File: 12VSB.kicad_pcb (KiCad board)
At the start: 4 copper layers, 24 parts, among them U1 FP6296

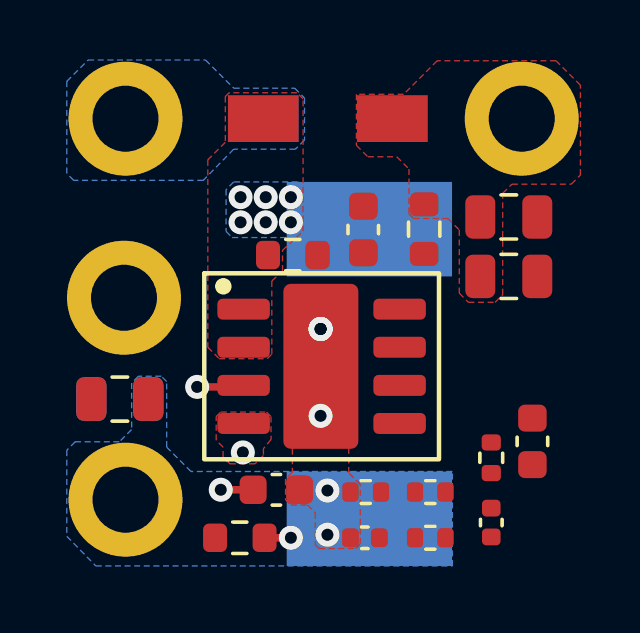
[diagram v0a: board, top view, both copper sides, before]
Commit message: Updated PCB Layout and Documentation
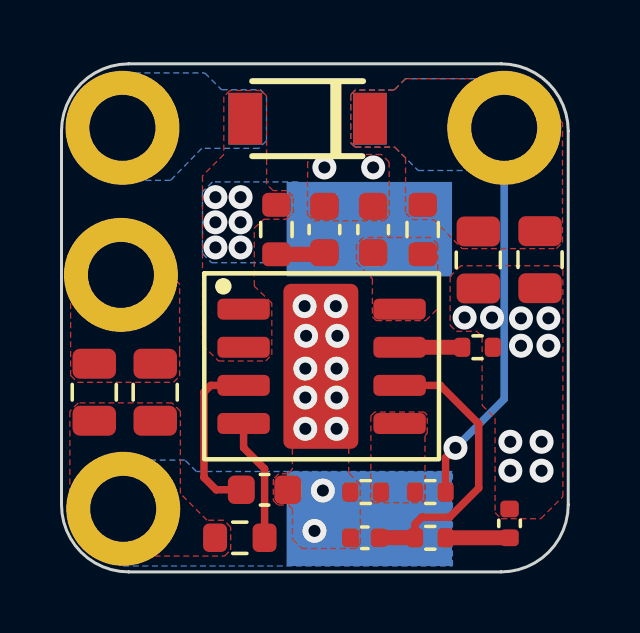
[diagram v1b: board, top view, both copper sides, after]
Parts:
- C2: moved to F.Cu
- moved C9 8.83 mm to (63.1, 58.1)
- moved R3 3.71 mm to (66.6, 62.0), turned to 0 degrees
- moved C5 1.76 mm to (68.7, 59.1), turned to -90 degrees
- moved C12 1.30 mm to (61.5, 58.1)
- moved C2 1.20 mm to (55.9, 63.5), turned to 90 degrees
- moved C6 1.15 mm to (66.6, 59.1), turned to -90 degrees
- moved R8 1.01 mm to (59.9, 58.1), turned to 90 degrees
- moved C1 0.88 mm to (53.8, 63.5), turned to 90 degrees
- moved H3 0.77 mm to (54.7, 59.6), turned to 90 degrees
- moved D1 0.67 mm to (60.9, 54.4)
- moved D2 0.67 mm to (60.9, 54.4)
- moved H4 0.66 mm to (67.5, 54.7)
- moved C4 0.61 mm to (67.7, 67.8)
- moved C3 0.39 mm to (59.5, 66.7)
- moved H1 0.32 mm to (54.8, 54.7)
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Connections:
- net GNDREF renamed GND
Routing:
- net 12VSB: track 0.00 -> 13.0 mm, vias 0 -> 1
- net Net-(U1-COMP): track 0.00 -> 9.58 mm
- net Net-(C4-Pad1): track 0.00 -> 2.13 mm
- net Net-(U1-OC): track 0.00 -> 2.09 mm
- net Net-(C12-Pad1): track 0.00 -> 1.62 mm
- net 5VSB: track 0.36 -> 1.72 mm
- net Net-(U1-EN): track 5.14 -> 4.26 mm, vias 2 -> 0
- net Net-(U1-VCC): track 6.40 -> 5.75 mm, vias 2 -> 0
- net GND: vias 5 -> 24
- added copper zone on B.Cu, net 12VSB
- added copper zone on F.Cu, net 5VSB
- added copper zone on In1.Cu, net GND
- added copper zone on In2.Cu, net GND
- added copper zone on F.Cu, net Net-(U1-FB)
- added copper zone on F.Cu, net Net-(U1-HVDD)
- removed copper zone on F.Cu, net Net-(U1-EN)
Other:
- board outline added: 16.9 x 16.9 mm
- board text added: "+12V"
- board text added: "+12VSB"
- board text added: "+5VSB"
- board text added: "GND"
